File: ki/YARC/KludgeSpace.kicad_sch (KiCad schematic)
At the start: 4 parts, among them J8 6-PIN FROM MCR, U100 74LS32, U101 74LS157, U96 74LS32

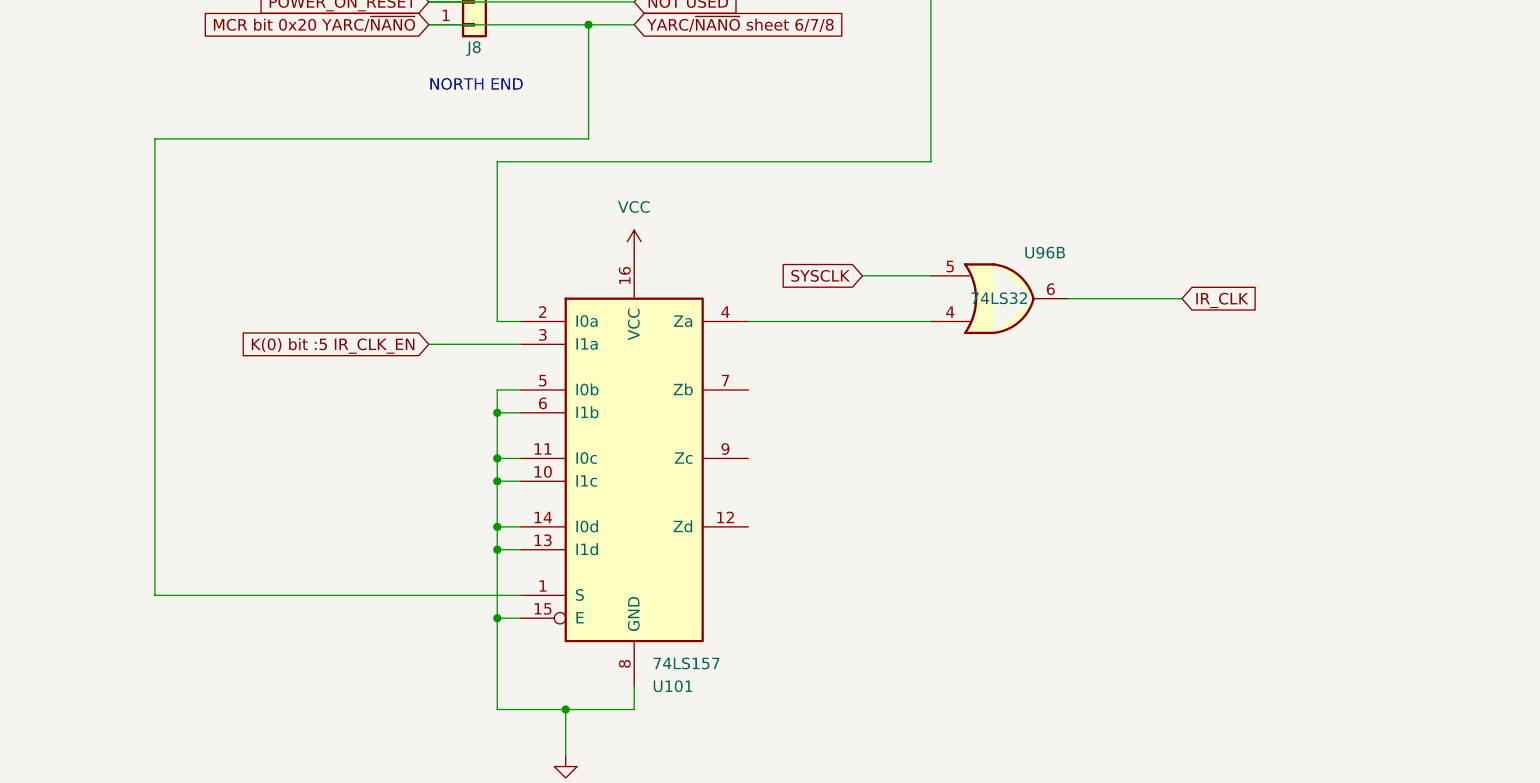
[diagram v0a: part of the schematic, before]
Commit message: Minor changes while wiring Port1 address transceiver
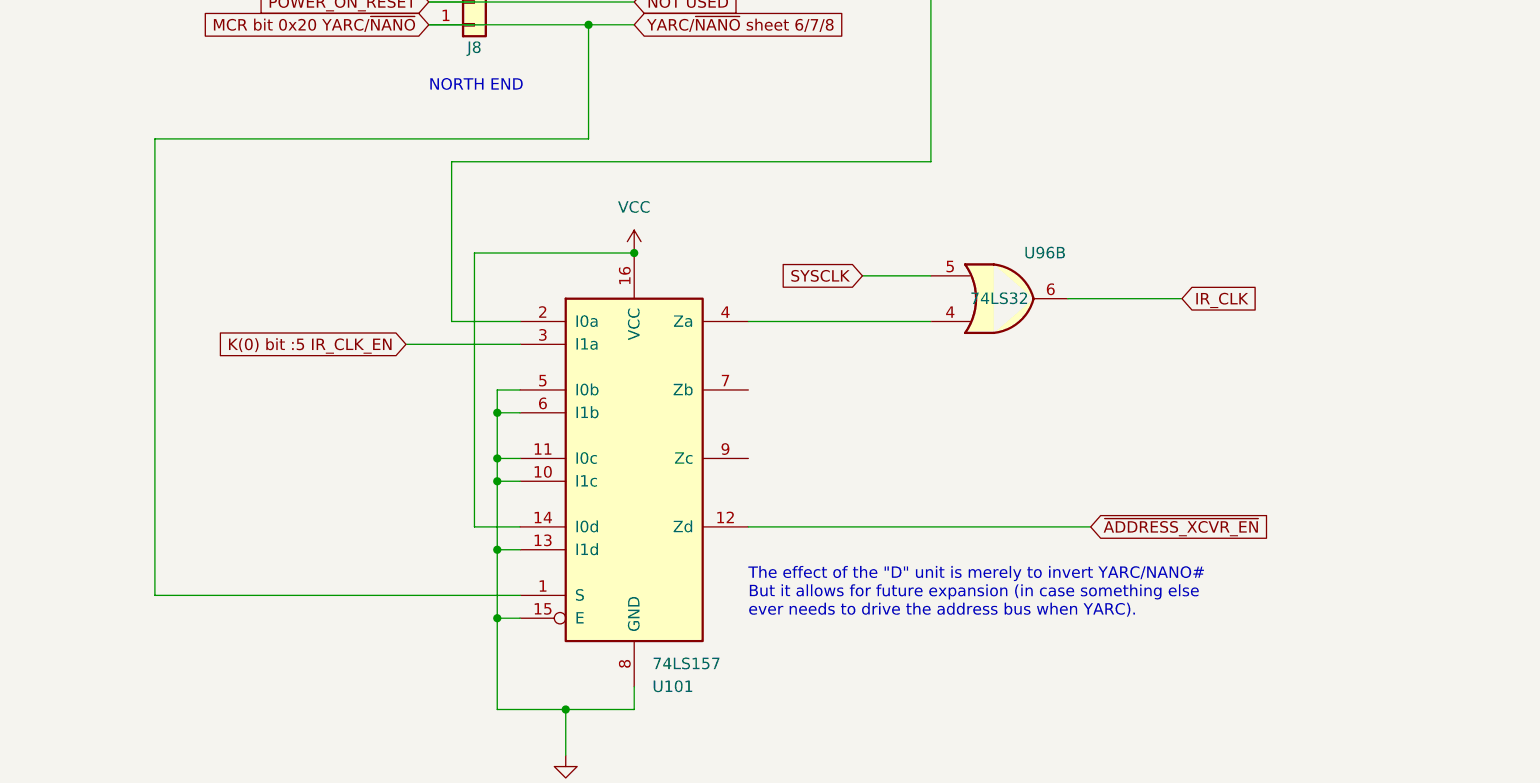
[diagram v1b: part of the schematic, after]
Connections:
- net GND: no longer U101.14 (I0d)
- net VCC: now also U101.14 (I0d)
- net ~{ADDRESS_XCVR_EN}: now reaches U101.12 (Zd)
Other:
- note added: "The effect of the "D" unit is merely to invert YARC/NANO# But it allows for future expansion (in case something else ever needs to drive the address bus when YARC)."
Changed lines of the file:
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@@
   (junction (at 63.5 119.38) (diameter 0) (color 0 0 0 0)
   )
+  (junction (at 78.74 78.74) (diameter 0) (color 0 0 0 0)
+  )
   (junction (at 63.5 101.6) (diameter 0) (color 0 0 0 0)
   )
@@
   (junction (at 63.5 104.14) (diameter 0) (color 0 0 0 0)
   )
+  (junction (at 63.5 111.76) (diameter 0) (color 0 0 0 0)
+  )
   (junction (at 73.66 53.34) (diameter 0) (color 0 0 0 0)
   )
-  (junction (at 63.5 111.76) (diameter 0) (color 0 0 0 0)
-  )
   (junction (at 71.12 129.54) (diameter 0) (color 0 0 0 0)
   )
-  (junction (at 63.5 109.22) (diameter 0) (color 0 0 0 0)
-  )
   (wire (pts (xy 104.14 81.28) (xy 111.76 81.28))
     (stroke (width 0) (type default) (color 0 0 0 0))
@@
     (stroke (width 0) (type default) (color 0 0 0 0))
   )
-  (wire (pts (xy 63.5 109.22) (xy 63.5 111.76))
-    (stroke (width 0) (type default) (color 0 0 0 0))
-  )
   (wire (pts (xy 66.04 101.6) (xy 63.5 101.6))
     (stroke (width 0) (type default) (color 0 0 0 0))
@@
     (stroke (width 0) (type default) (color 0 0 0 0))
   )
-  (wire (pts (xy 66.04 86.36) (xy 63.5 86.36))
+  (wire (pts (xy 58.42 86.36) (xy 66.04 86.36))
     (stroke (width 0) (type default) (color 0 0 0 0))
   )
@@
     (stroke (width 0) (type default) (color 0 0 0 0))
   )
-  (wire (pts (xy 63.5 119.38) (xy 63.5 111.76))
-    (stroke (width 0) (type default) (color 0 0 0 0))
-  )
   (wire (pts (xy 111.76 68.58) (xy 111.76 43.18))
     (stroke (width 0) (type default) (color 0 0 0 0))
   )
+  (wire (pts (xy 91.44 109.22) (xy 129.54 109.22))
+    (stroke (width 0) (type default) (color 0 0 0 0))
+  )
   (wire (pts (xy 73.66 53.34) (xy 78.74 53.34))
     (stroke (width 0) (type default) (color 0 0 0 0))
@@
     (stroke (width 0) (type default) (color 0 0 0 0))
   )
-  (wire (pts (xy 63.5 86.36) (xy 63.5 68.58))
-    (stroke (width 0) (type default) (color 0 0 0 0))
-  )
   (wire (pts (xy 55.88 53.34) (xy 73.66 53.34))
     (stroke (width 0) (type default) (color 0 0 0 0))
   )
+  (wire (pts (xy 60.96 109.22) (xy 60.96 78.74))
+    (stroke (width 0) (type default) (color 0 0 0 0))
+  )
   (wire (pts (xy 63.5 96.52) (xy 63.5 101.6))
     (stroke (width 0) (type default) (color 0 0 0 0))
@@
     (stroke (width 0) (type default) (color 0 0 0 0))
   )
+  (wire (pts (xy 91.44 86.36) (xy 111.76 86.36))
+    (stroke (width 0) (type default) (color 0 0 0 0))
+  )
+  (wire (pts (xy 58.42 68.58) (xy 58.42 86.36))
+    (stroke (width 0) (type default) (color 0 0 0 0))
+  )
+  (wire (pts (xy 78.74 48.26) (xy 55.88 48.26))
+    (stroke (width 0) (type default) (color 0 0 0 0))
+  )
   (wire (pts (xy 66.04 111.76) (xy 63.5 111.76))
     (stroke (width 0) (type default) (color 0 0 0 0))
   )
-  (wire (pts (xy 91.44 86.36) (xy 111.76 86.36))
-    (stroke (width 0) (type default) (color 0 0 0 0))
-  )
-  (wire (pts (xy 78.74 48.26) (xy 55.88 48.26))
-    (stroke (width 0) (type default) (color 0 0 0 0))
-  )
   (wire (pts (xy 78.74 50.8) (xy 55.88 50.8))
     (stroke (width 0) (type default) (color 0 0 0 0))
@@
     (stroke (width 0) (type default) (color 0 0 0 0))
   )
-  (wire (pts (xy 66.04 88.9) (xy 55.88 88.9))
+  (wire (pts (xy 66.04 88.9) (xy 53.34 88.9))
     (stroke (width 0) (type default) (color 0 0 0 0))
   )
@@
     (stroke (width 0) (type default) (color 0 0 0 0))
   )
+  (wire (pts (xy 63.5 111.76) (xy 63.5 119.38))
+    (stroke (width 0) (type default) (color 0 0 0 0))
+  )
   (wire (pts (xy 127 83.82) (xy 139.7 83.82))
     (stroke (width 0) (type default) (color 0 0 0 0))
@@
     (stroke (width 0) (type default) (color 0 0 0 0))
   )
-  (wire (pts (xy 66.04 109.22) (xy 63.5 109.22))
-    (stroke (width 0) (type default) (color 0 0 0 0))
-  )
   (wire (pts (xy 78.74 45.72) (xy 55.88 45.72))
     (stroke (width 0) (type default) (color 0 0 0 0))
@@
     (stroke (width 0) (type default) (color 0 0 0 0))
   )
+  (wire (pts (xy 66.04 109.22) (xy 60.96 109.22))
+    (stroke (width 0) (type default) (color 0 0 0 0))
+  )
+  (wire (pts (xy 60.96 78.74) (xy 78.74 78.74))
+    (stroke (width 0) (type default) (color 0 0 0 0))
+  )
   (wire (pts (xy 71.12 129.54) (xy 78.74 129.54))
     (stroke (width 0) (type default) (color 0 0 0 0))
   )
-  (wire (pts (xy 63.5 104.14) (xy 63.5 109.22))
+  (wire (pts (xy 63.5 104.14) (xy 63.5 111.76))
     (stroke (width 0) (type default) (color 0 0 0 0))
   )
@@
     (stroke (width 0) (type default) (color 0 0 0 0))
   )
-  (wire (pts (xy 63.5 68.58) (xy 111.76 68.58))
+  (wire (pts (xy 58.42 68.58) (xy 111.76 68.58))
     (stroke (width 0) (type default) (color 0 0 0 0))
   )
@@
   )
   (text "NORTH END" (at 55.88 60.96 0)
+    (effects (font (size 1.27 1.27)) (justify left bottom))
+  )
+  (text "The effect of the \"D\" unit is merely to invert YARC/NANO#\nBut it allows for future expansion (in case something else\never needs to drive the address bus when YARC)."
+    (at 91.44 119.38 0)
     (effects (font (size 1.27 1.27)) (justify left bottom))
   )
@@
     )
   )
-  (global_label "K(0) bit :5 IR_CLK_EN" (shape input) (at 55.88 88.9 180) (fields_autoplaced)
+  (global_label "K(0) bit :5 IR_CLK_EN" (shape input) (at 53.34 88.9 180) (fields_autoplaced)
     (effects (font (size 1.27 1.27)) (justify right))
-    (property "Intersheet References" "${INTERSHEET_REFS}" (id 0) (at 32.2398 88.8206 0)
+    (property "Intersheet References" "${INTERSHEET_REFS}" (id 0) (at 29.6998 88.8206 0)
       (effects (font (size 1.27 1.27)) (justify right) hide)
     )
@@
     )
   )
+  (global_label "~{ADDRESS_XCVR_EN}" (shape input) (at 129.54 109.22 0) (fields_autoplaced)
+    (effects (font (size 1.27 1.27)) (justify left))
+    (property "Intersheet References" "${INTERSHEET_REFS}" (id 0) (at 149.6726 109.1406 0)
+      (effects (font (size 1.27 1.27)) (justify left) hide)
+    )
+  )
